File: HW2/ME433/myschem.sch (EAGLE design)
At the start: 1 part

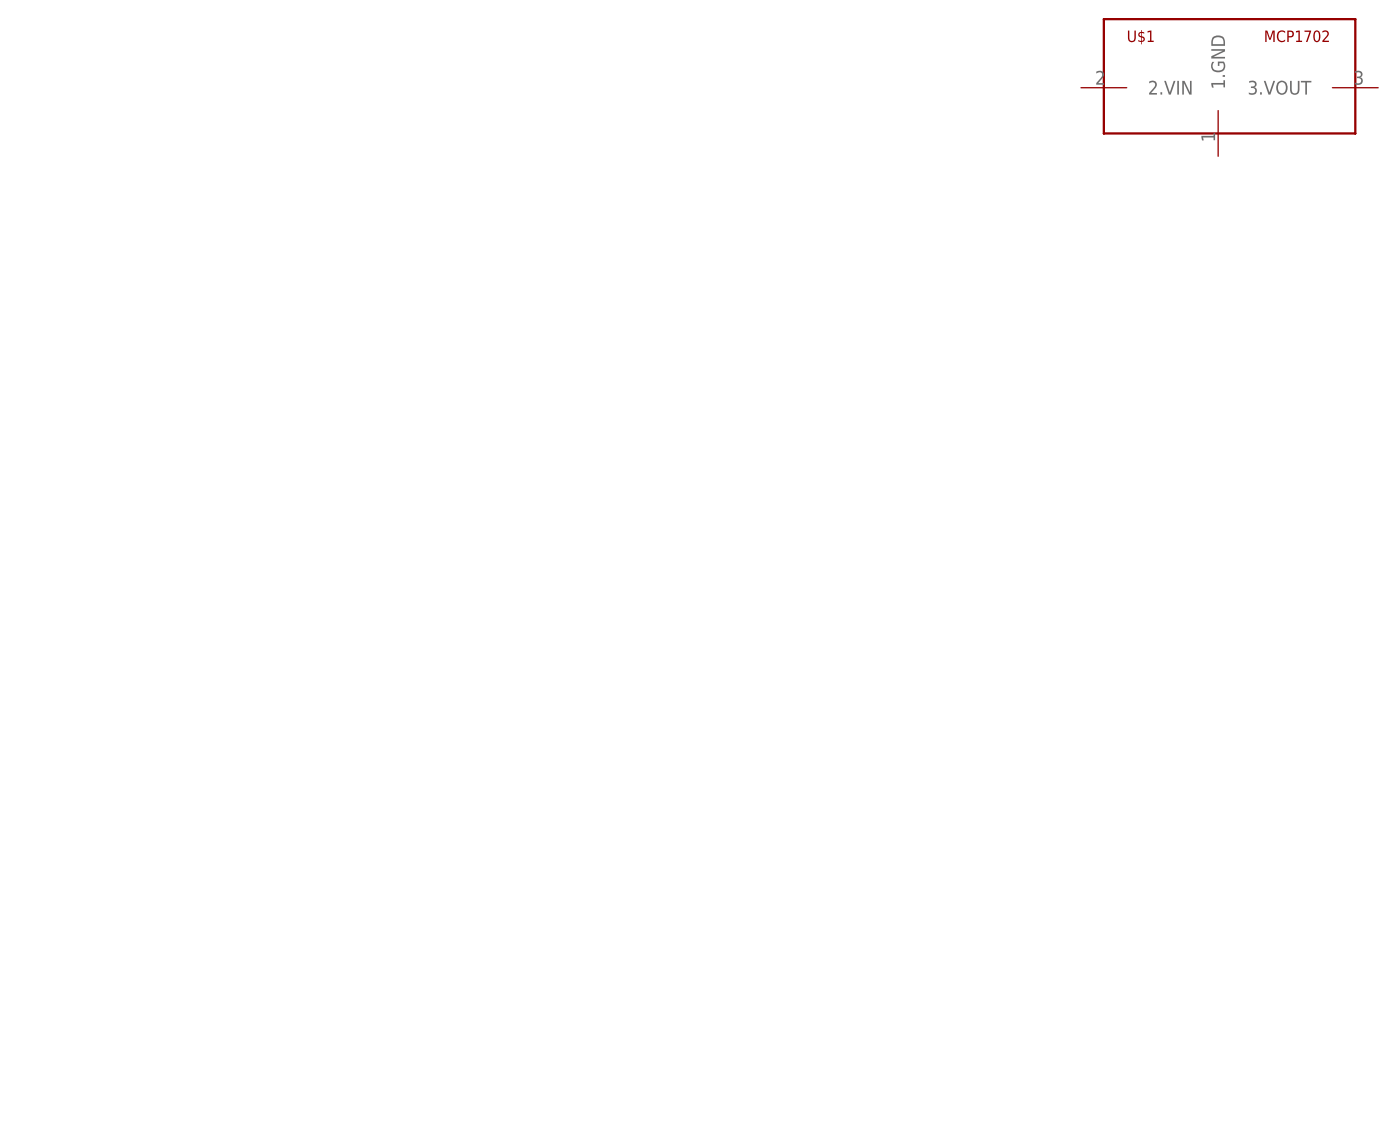
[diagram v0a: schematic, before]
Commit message: Finished PCB design.
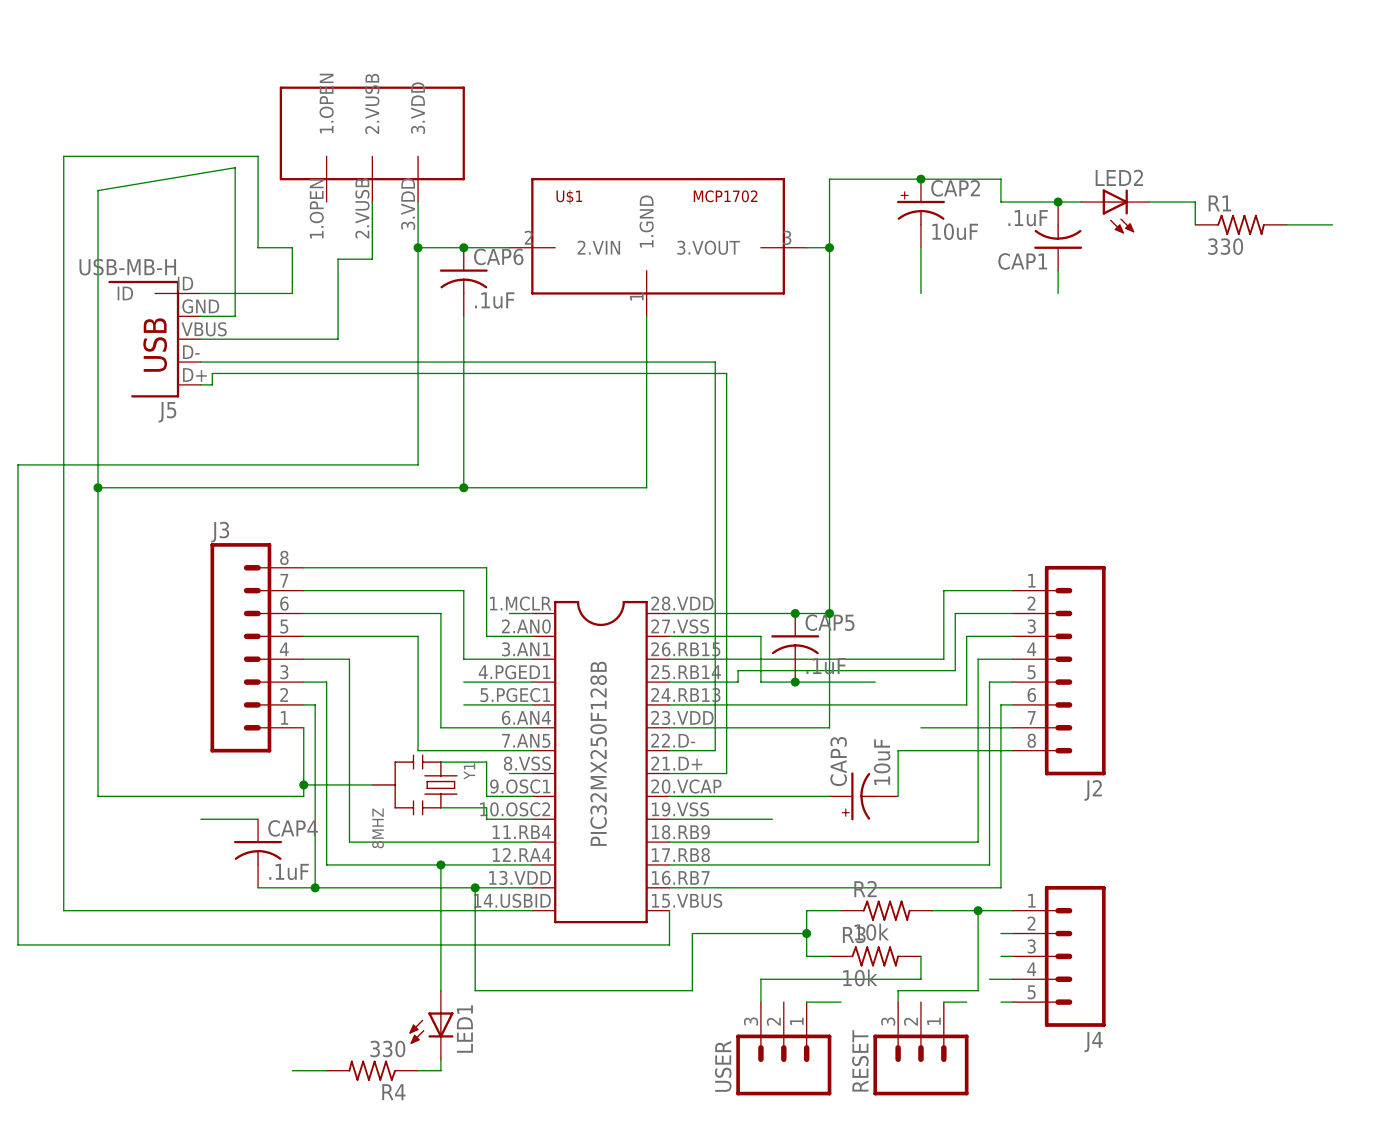
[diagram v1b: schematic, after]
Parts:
- added CAP1, CAP4, CAP5, CAP6: .1uF, mylib:C-US025-024X044
- added CAP2, CAP3: 10uF, mylib:CPOL-USB45181B
- added J2, J3: (no value), mylib:M08
- added J4: (no value), mylib:M05PTH
- added J5: USB-MB-H, mylib:USB-MB-H
- added LED1, LED2: (no value), mylib:LED3MM
- added PIC32MX250F128B: (no value), mylib:DIL28-3
- added R1, R4: 330, mylib:R-US_0207/10
- added R2, R3: 10k, mylib:R-US_0207/10
- added RESET, USER: (no value), mylib:M03PTH
- added U$2: SLIDE-SWTICH, mylib:SLIDE-SWTICH
- added Y1: 8MHZ, mylib:DIP-CERAMIC-RESONATOR/-OSCILLATOR-8MHZ(3P-2.5-8X3MM)
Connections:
- new net GND: CAP1.1, CAP2.-, CAP3.-, CAP4.1, CAP5.2, CAP6.2, J2.8, J3.1, J4.3, J5.GND, PIC32MX250F128B.19, PIC32MX250F128B.27, PIC32MX250F128B.8, R1.2, R4.2, RESET.1, U$1.1.GND, USER.1, Y1.2
- new net MCLR: J4.1, PIC32MX250F128B.1, R2.2, RESET.3
- new net N$1: J3.8, PIC32MX250F128B.2
- new net N$10: PIC32MX250F128B.10, Y1.3
- new net N$11: LED2.C, R1.1
- new net N$12: J5.VBUS, U$2.2.VUSB
- new net N$14: J2.6, PIC32MX250F128B.16
- new net N$15: LED1.C, R4.1
- new net N$17: J2.1, PIC32MX250F128B.26
- new net N$18: J2.2, PIC32MX250F128B.25
- new net N$19: J2.3, PIC32MX250F128B.24
- new net N$2: J3.7, PIC32MX250F128B.3
- new net N$20: J2.4, PIC32MX250F128B.18
- new net N$21: J2.5, PIC32MX250F128B.17
- new net N$22: CAP3.+, PIC32MX250F128B.20
- new net N$3: J3.6, PIC32MX250F128B.6
- new net N$4: J3.5, PIC32MX250F128B.7
- new net N$5: J5.D-, PIC32MX250F128B.22
- new net N$6: J5.D+, PIC32MX250F128B.21
- new net N$7: J3.3, LED1.A, PIC32MX250F128B.12
- new net N$8: J5.ID, PIC32MX250F128B.14
- new net N$9: PIC32MX250F128B.9, Y1.1
- new net PGEC1: J4.5, PIC32MX250F128B.5
- new net PGED1: J4.4, PIC32MX250F128B.4
- new net USER: J3.4, PIC32MX250F128B.11, R3.2, USER.3
- new net VBUS: CAP6.1, J2.7, PIC32MX250F128B.15, U$1.2.VIN, U$2.3.VDD
- new net VDD: CAP1.2, CAP2.+, CAP4.2, CAP5.1, J3.2, J4.2, LED2.A, PIC32MX250F128B.13, PIC32MX250F128B.23, PIC32MX250F128B.28, R2.1, R3.1, U$1.3.VOUT
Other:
- moved on the sheet: U$1
